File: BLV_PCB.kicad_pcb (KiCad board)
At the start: 4 copper layers, 90 x 90 mm, 95 parts, among them J1 JST-PH, J10 USB_C_USB2.0_16P, J11 Micro_SD_Card, J12 duPont, J2 JST-PH, J3 JST-PH, J4 duPont, J5 duPont, J6 duPont, J8 USB_C_USB2.0_16P, Q1 Si2301CDS, Q2 Si2301CDS, SW11 SW_QSPI, SW12 SW_RUN, SW3 SW_GNSS, U11 W25Q128JVS, U12 RP2350_60QFN, U3 TPS63001DRCR, U4 BH-18650-A6AJ012, U5 E32-400M30S, U6 NEO-M9N, Y11 ABM8_262_T3

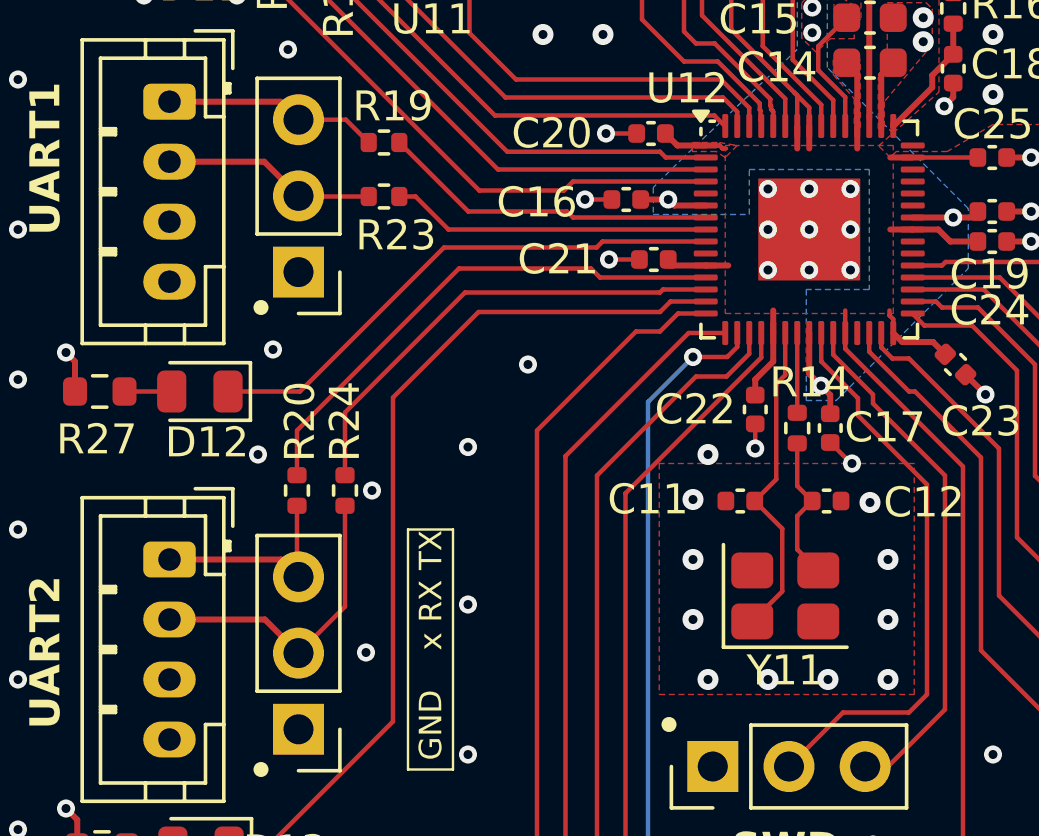
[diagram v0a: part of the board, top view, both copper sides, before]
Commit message: v1.0.1 - RF Fix
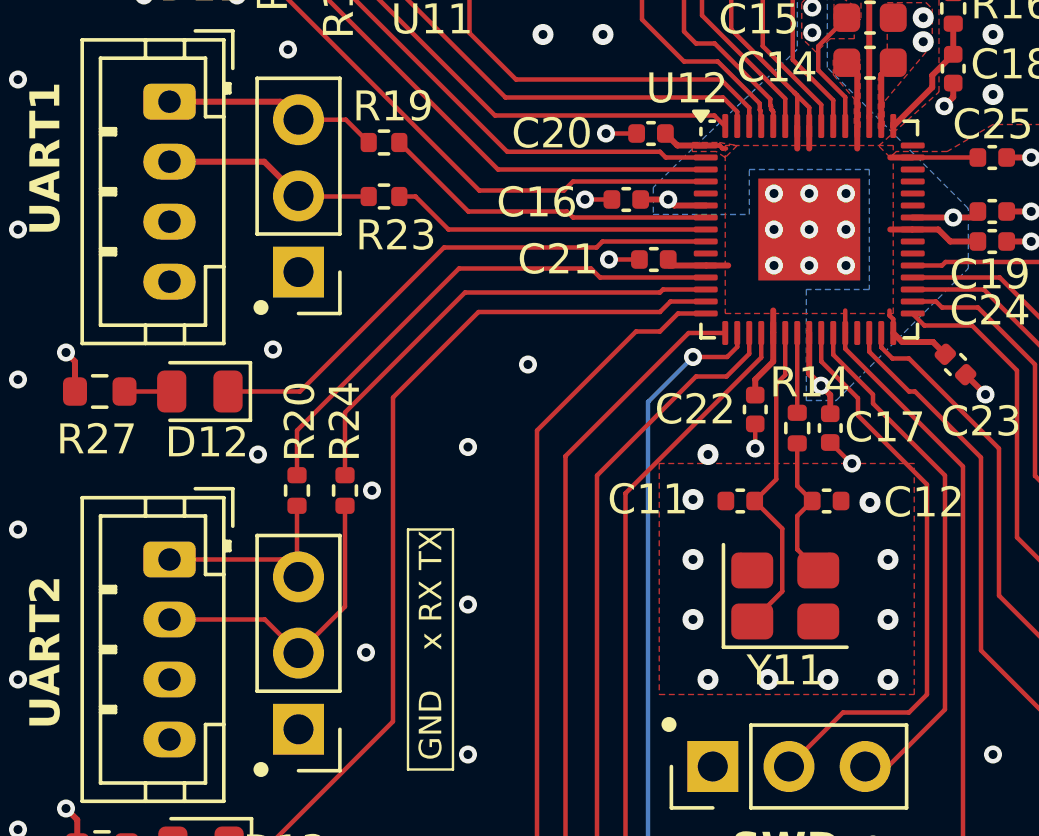
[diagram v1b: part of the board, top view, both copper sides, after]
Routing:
- added copper zone on In1.Cu, net +1V1
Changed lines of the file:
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@@
 	)
 	(via
-		(at 158.75 69.65)
+		(at 158.6 69.8)
 		(size 0.6)
 		(drill 0.3)
@@
 	)
 	(via
-		(at 156 71)
+		(at 156.2 71)
 		(size 0.6)
 		(drill 0.3)
@@
 	)
 	(via
-		(at 156 72.35)
+		(at 156.2 72.2)
 		(size 0.6)
 		(drill 0.3)
@@
 	)
 	(via
-		(at 158.75 72.35)
+		(at 158.6 72.2)
 		(size 0.6)
 		(drill 0.3)
@@
 	)
 	(via
-		(at 156 69.65)
+		(at 156.2 69.8)
 		(size 0.6)
 		(drill 0.3)
@@
 	)
 	(via
-		(at 157.375 69.65)
+		(at 157.375 69.8)
 		(size 0.6)
 		(drill 0.3)
@@
 	)
 	(via
-		(at 158.75 71)
+		(at 158.6 71)
 		(size 0.6)
 		(drill 0.3)
@@
 	)
 	(via
-		(at 157.375 72.35)
+		(at 157.375 72.2)
 		(size 0.6)
 		(drill 0.3)
@@
 		(start 139.23 84)
 		(end 140.35 85.12)
-		(width 0.2)
+		(width 0.15)
 		(layer "F.Cu")
 		(net 32)
@@
 		(start 136.5 84)
 		(end 139.23 84)
-		(width 0.2)
+		(width 0.15)
 		(layer "F.Cu")
 		(net 32)
 	)
 	(segment
-		(start 140.3 82.53)
-		(end 140.35 82.58)
+		(start 136.5 82)
+		(end 139.77 82)
 		(width 0.15)
 		(layer "F.Cu")
@@
 	)
 	(segment
-		(start 139.77 82)
-		(end 140.35 82.58)
-		(width 0.2)
-		(layer "F.Cu")
-		(net 33)
-	)
-	(segment
-		(start 136.5 82)
+		(start 140.35 82.58)
 		(end 139.77 82)
-		(width 0.2)
+		(width 0.15)
 		(layer "F.Cu")
 		(net 33)
@@
 	)
 	(zone
-		(net 3)
-		(net_name "+1V1")
+		(net 25)
+		(net_name "GND")
 		(layer "B.Cu")
+		(name "GND")
 		(hatch edge 0.5)
-		(priority 12)
-		(connect_pads
+		(connect_pads yes
 			(clearance 0.3)
 		)
@@
 			(thermal_gap 0.5)
 			(thermal_bridge_width 0.5)
+			(smoothing fillet)
+			(radius 0.1)
 		)
 		(polygon
 			(pts
-				(xy 156.975 63.1) (xy 156.975 64.994872) (xy 153.175 68.6) (xy 152.175 69.6) (xy 152.175 70.5) (xy 155.375 70.5)
-				(xy 155.375 69) (xy 159.375 69) (xy 159.375 73) (xy 157.275 73) (xy 157.275 76.7) (xy 158.275 76.7)
-				(xy 162.675 72.3) (xy 162.675 70.3) (xy 157.975 65.6) (xy 157.975 63.1)
+				(xy 130 40) (xy 220 40) (xy 220 130) (xy 130 130)
 			)
 		)
 	)
 	(zone
-		(net 25)
-		(net_name "GND")
-		(layer "B.Cu")
-		(name "GND")
+		(net 3)
+		(net_name "+1V1")
+		(layers "B.Cu" "In1.Cu")
 		(hatch edge 0.5)
-		(connect_pads yes
+		(priority 12)
+		(connect_pads
 			(clearance 0.3)
 		)
@@
 			(thermal_gap 0.5)
 			(thermal_bridge_width 0.5)
-			(smoothing fillet)
-			(radius 0.1)
 		)
 		(polygon
 			(pts
-				(xy 130 40) (xy 220 40) (xy 220 130) (xy 130 130)
+				(xy 156.975 63.1) (xy 156.975 64.994872) (xy 153.175 68.6) (xy 152.175 69.6) (xy 152.175 70.5) (xy 155.375 70.5)
+				(xy 155.375 69) (xy 159.375 69) (xy 159.375 73) (xy 157.275 73) (xy 157.275 76.7) (xy 158.275 76.7)
+				(xy 162.675 72.3) (xy 162.675 70.3) (xy 157.975 65.6) (xy 157.975 63.1)
 			)
 		)
